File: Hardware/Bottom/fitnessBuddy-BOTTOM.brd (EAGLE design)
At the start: 33 x 33 mm, 47 parts, among them U4 PCF8523

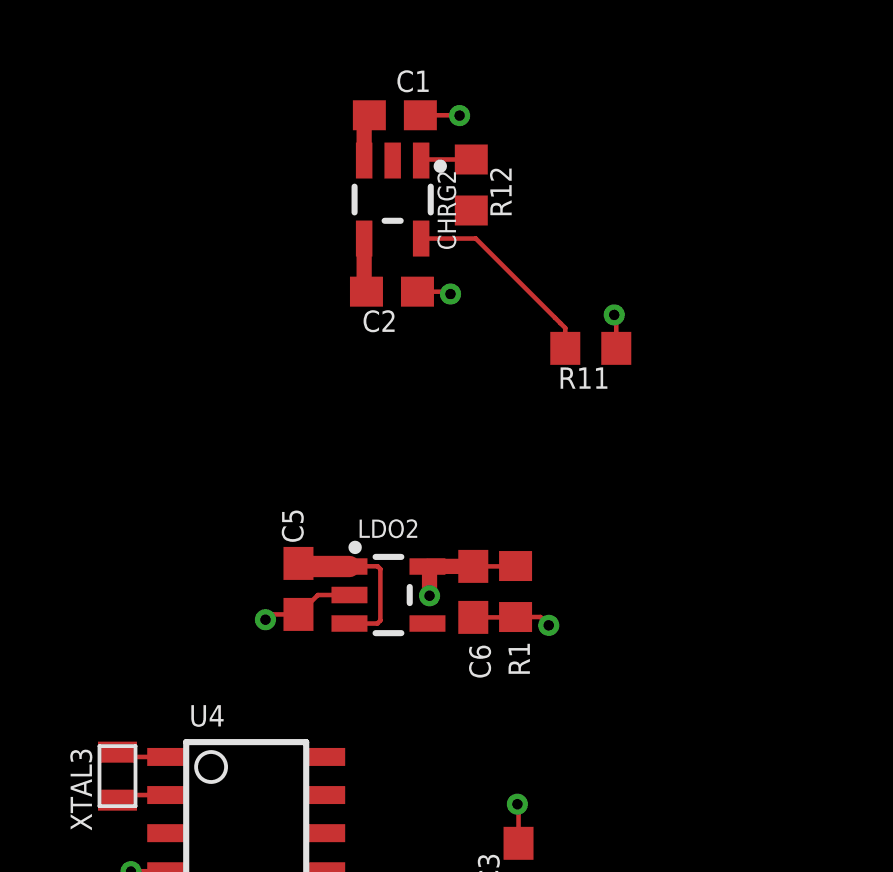
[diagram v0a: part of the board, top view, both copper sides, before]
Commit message: organized top board
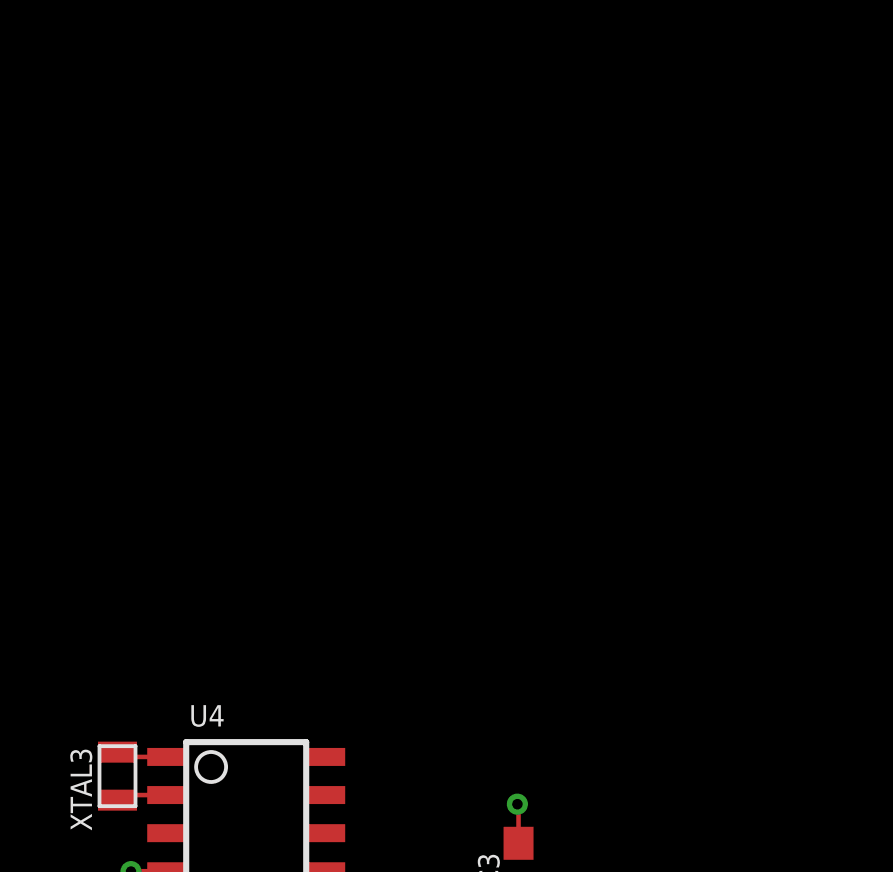
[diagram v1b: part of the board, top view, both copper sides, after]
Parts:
- removed C1, C2: 4.7u, LinnesLab-Passives:C0603
- removed C5, C6: 1u, LinnesLab-Passives:C0603
- removed CHRG2: MCP73831, LinnesLab-Power:SOT23-5
- removed LDO2: MIC5504, LinnesLab-Power:SOT23-5
- removed R1, R12: 100k, LinnesLab-Passives:R0603
- removed R11: (no value), LinnesLab-Passives:R0603
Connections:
- removed net D27/CHRG.STATUS: CHRG2.1, R12.1
- removed net N$4: CHRG2.5, R11.2
- removed net VIN: C2.2, C5.2, CHRG2.4, LDO2.1, LDO2.3, R12.2
- removed net VLIPO: C1.1, CHRG2.3
- net 3.3V: no longer C6.1, LDO2.5, R1.2
- net GND: no longer C1.2, C2.1, C5.1, C6.2, CHRG2.2, LDO2.2, R1.1, R11.1
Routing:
- net GND: track 39.5 -> 30.1 mm, vias 22 -> 17
- net VIN: track 7.40 -> 0.00 mm
- net N$4: track 6.72 -> 0.00 mm
- net 3.3V: track 5.60 -> 1.32 mm, vias 1 -> 0
- net D27/CHRG.STATUS: track 1.69 -> 0.00 mm
- net VLIPO: track 1.58 -> 0.00 mm
